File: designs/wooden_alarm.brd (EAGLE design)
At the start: 47.8 x 53 mm, 20 parts, among them IC1 ESP-12E/F

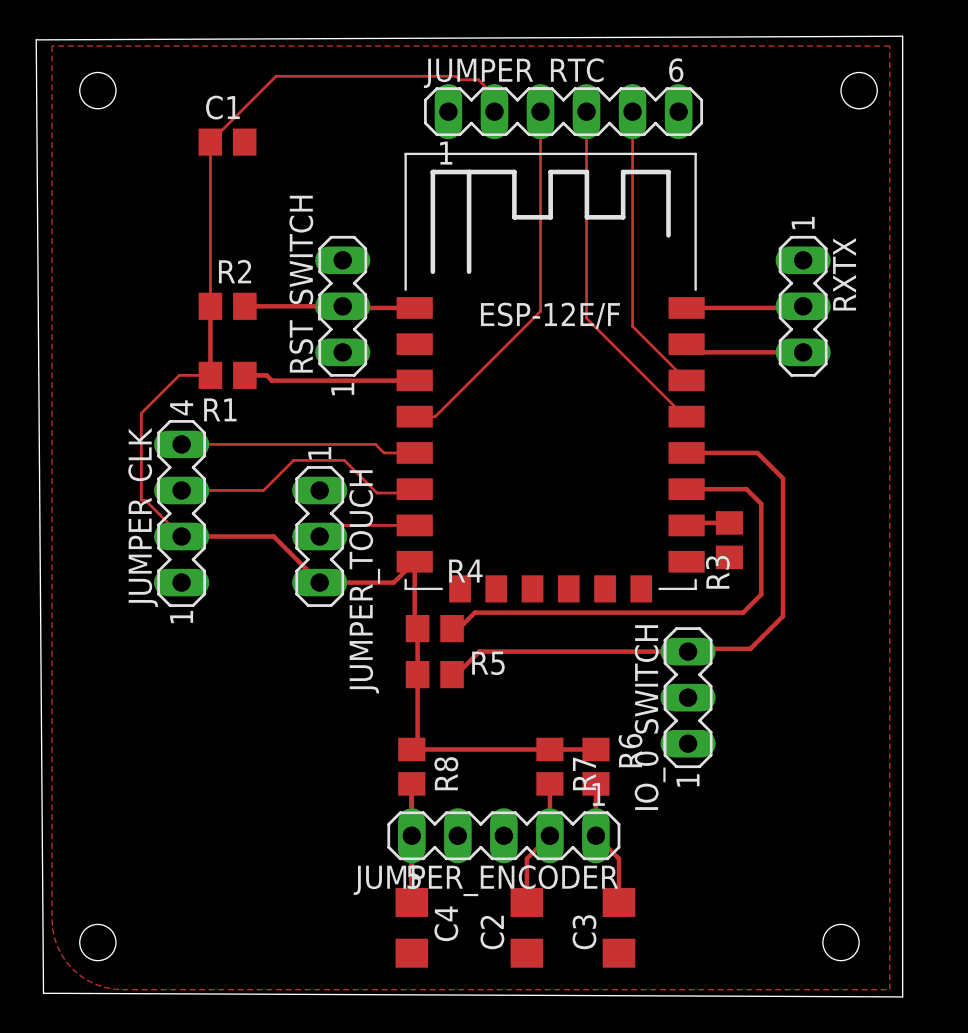
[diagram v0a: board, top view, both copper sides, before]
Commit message: final changes v1 design
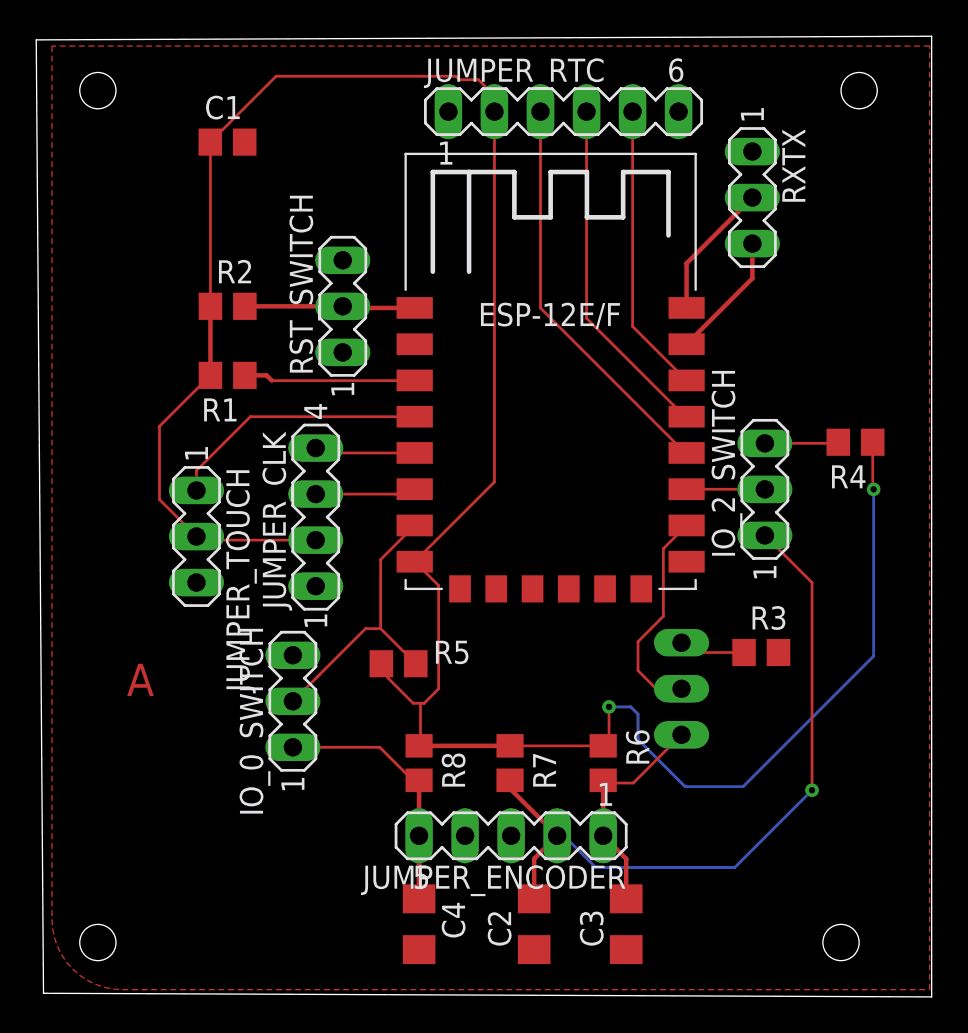
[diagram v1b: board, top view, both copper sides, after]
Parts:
- added IO_15_SWITCH, IO_2_SWITCH: (no value), con-lstb:MA03-1
- moved R4 25.4 mm to (44.8, 30.6), turned to 180 degrees
- moved IO_0_SWITCH 21.8 mm to (13.8, 16.3)
- moved JUMPER_CLK 7.40 mm to (15.0, 26.5)
- moved JUMPER_TOUCH 6.80 mm to (8.44, 25.4)
- moved RXTX 6.62 mm to (39.1, 44.1)
- moved R3 6.44 mm to (39.6, 19.0), turned to 0 degrees
- moved R7 2.21 mm to (25.7, 12.9)
- moved R5 2.09 mm to (19.6, 18.4)
- moved R6 0.45 mm to (30.9, 12.9)
- moved R8 0.45 mm to (20.7, 12.9)
- moved C2 0.45 mm to (27.1, 4.01)
- moved C3 0.45 mm to (32.1, 4.01)
- moved C4 0.45 mm to (20.7, 4.01)
- moved JUMPER_ENCODER 0.40 mm to (25.8, 8.89)
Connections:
- removed net N$8: IC1.IO0, IO_0_SWITCH.3, R5.2
- new net N$2: IO_2_SWITCH.3, R4.2
- new net N$5: IO_15_SWITCH.3, R3.1
- new net SWITCH_PIN: IC1.IO13, IO_0_SWITCH.2, R5.2
- net CCW: now also IO_2_SWITCH.1
- net CW: now also IO_15_SWITCH.1
- net GND: now also IO_0_SWITCH.3, JUMPER_TOUCH.3, R3.2; no longer IO_0_SWITCH.2, JUMPER_TOUCH.1, R3.1
- net N$3: now also IO_15_SWITCH.2; no longer R3.2
- net N$7: now also IO_2_SWITCH.2; no longer R4.2
- net SQW: now also IC1.IO0; no longer IC1.IO16
- net SWITCH: now also IO_0_SWITCH.1
- net TOUCH_IO: now also IC1.IO16, JUMPER_TOUCH.1; no longer IC1.IO13, JUMPER_TOUCH.2
- net VCC: now also JUMPER_TOUCH.2; no longer JUMPER_TOUCH.3
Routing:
- net VCC: track 79.0 -> 134.7 mm, vias 0 -> 2
- net N$8: track 33.1 -> 0.00 mm
- net CCW: track 7.07 -> 39.8 mm, vias 0 -> 1
- net N$7: track 27.3 -> 4.32 mm
- net SWITCH_PIN: track 0.00 -> 15.7 mm
- net N$3: track 2.42 -> 11.9 mm
- net TOUCH_IO: track 5.49 -> 14.4 mm
- net DIO_DISPLAY: track 14.4 -> 5.57 mm
- net CLK_DISPLAY: track 13.1 -> 5.57 mm
- net CW: track 7.07 -> 12.5 mm
- net SWITCH: track 13.1 -> 17.9 mm
- net N$2: track 0.00 -> 4.07 mm
- net N$5: track 0.00 -> 3.67 mm
- net SQW: track 20.4 -> 22.2 mm
- net TX: track 6.47 -> 7.59 mm
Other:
- board size 47.8 x 53 mm -> 49.4 x 53 mm
- board text added: "A"
